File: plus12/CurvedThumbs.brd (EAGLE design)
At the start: 123.8 x 54 mm, 14 parts

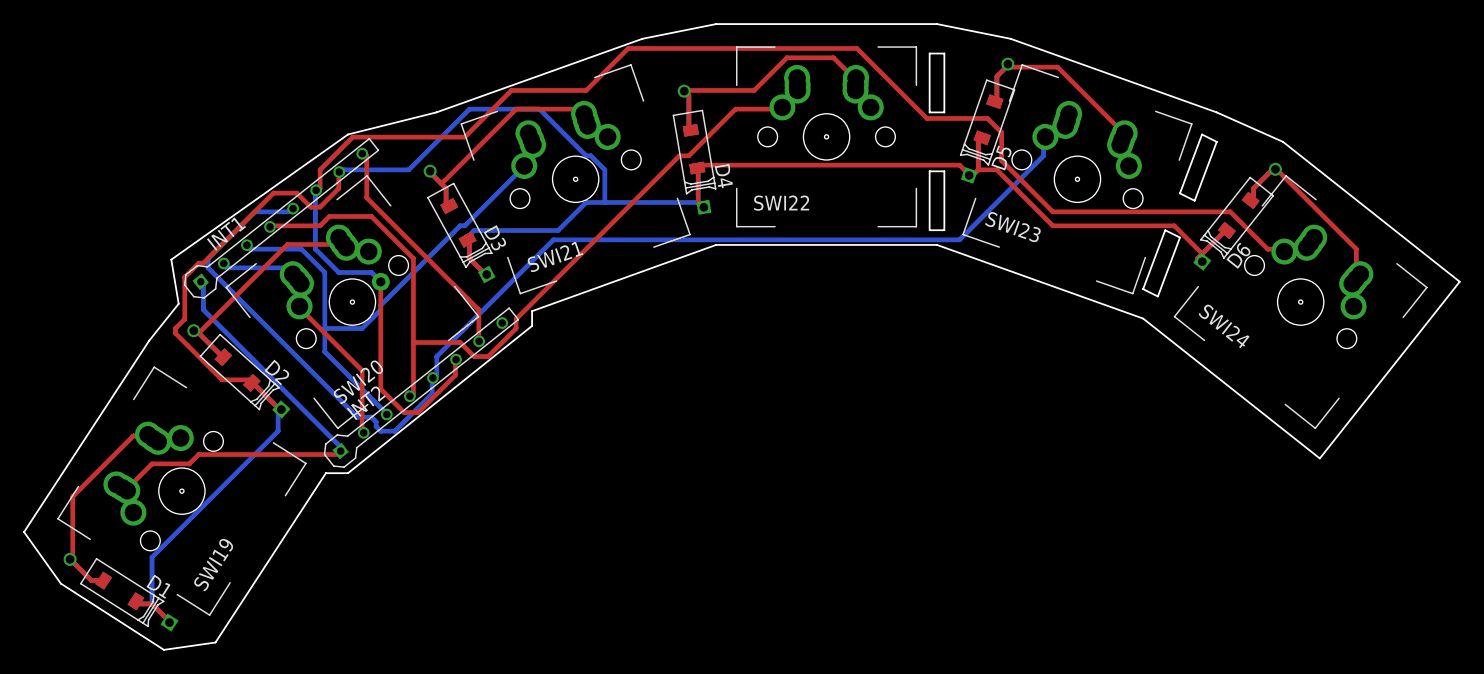
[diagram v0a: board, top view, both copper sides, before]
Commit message: Kobe beefing it up
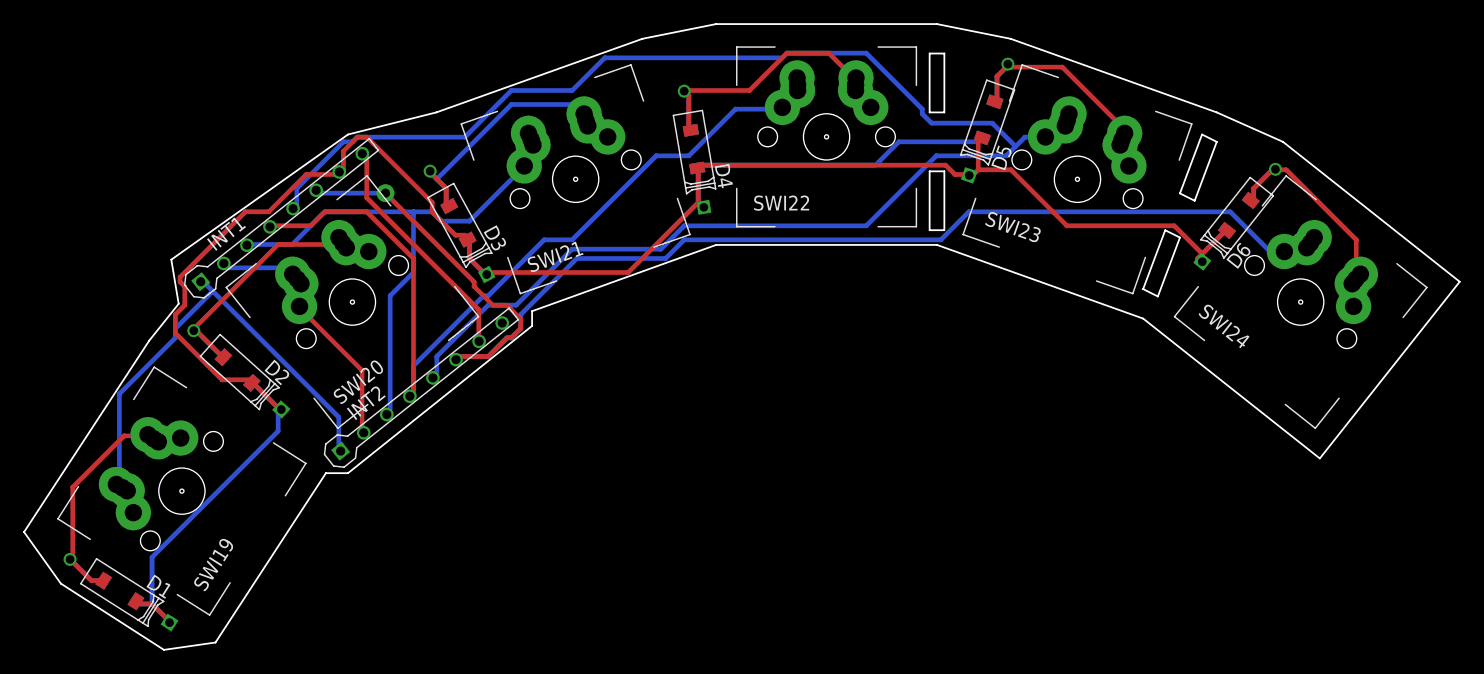
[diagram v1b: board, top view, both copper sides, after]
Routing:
- net N$11: track 106.0 -> 138.0 mm
- net N$12: track 133.6 -> 112.1 mm
- net N$13: track 197.9 -> 205.5 mm
- net N$10: track 72.4 -> 74.5 mm
- net N$8: track 24.1 -> 25.5 mm
- net N$7: track 44.9 -> 44.1 mm
- net N$3: track 22.4 -> 23.0 mm
- net N$5: track 20.8 -> 21.4 mm
